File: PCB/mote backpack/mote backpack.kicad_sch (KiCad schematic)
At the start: 15 parts, among them J1 DF17_2.0_-30DP-0.5V_57_, J2 73251-1350, J3 Micro_SD_Card_Det2, J4 Conn_01x06_Socket, U1 MAX3232, U3 ADAFRUIT_QT_PY

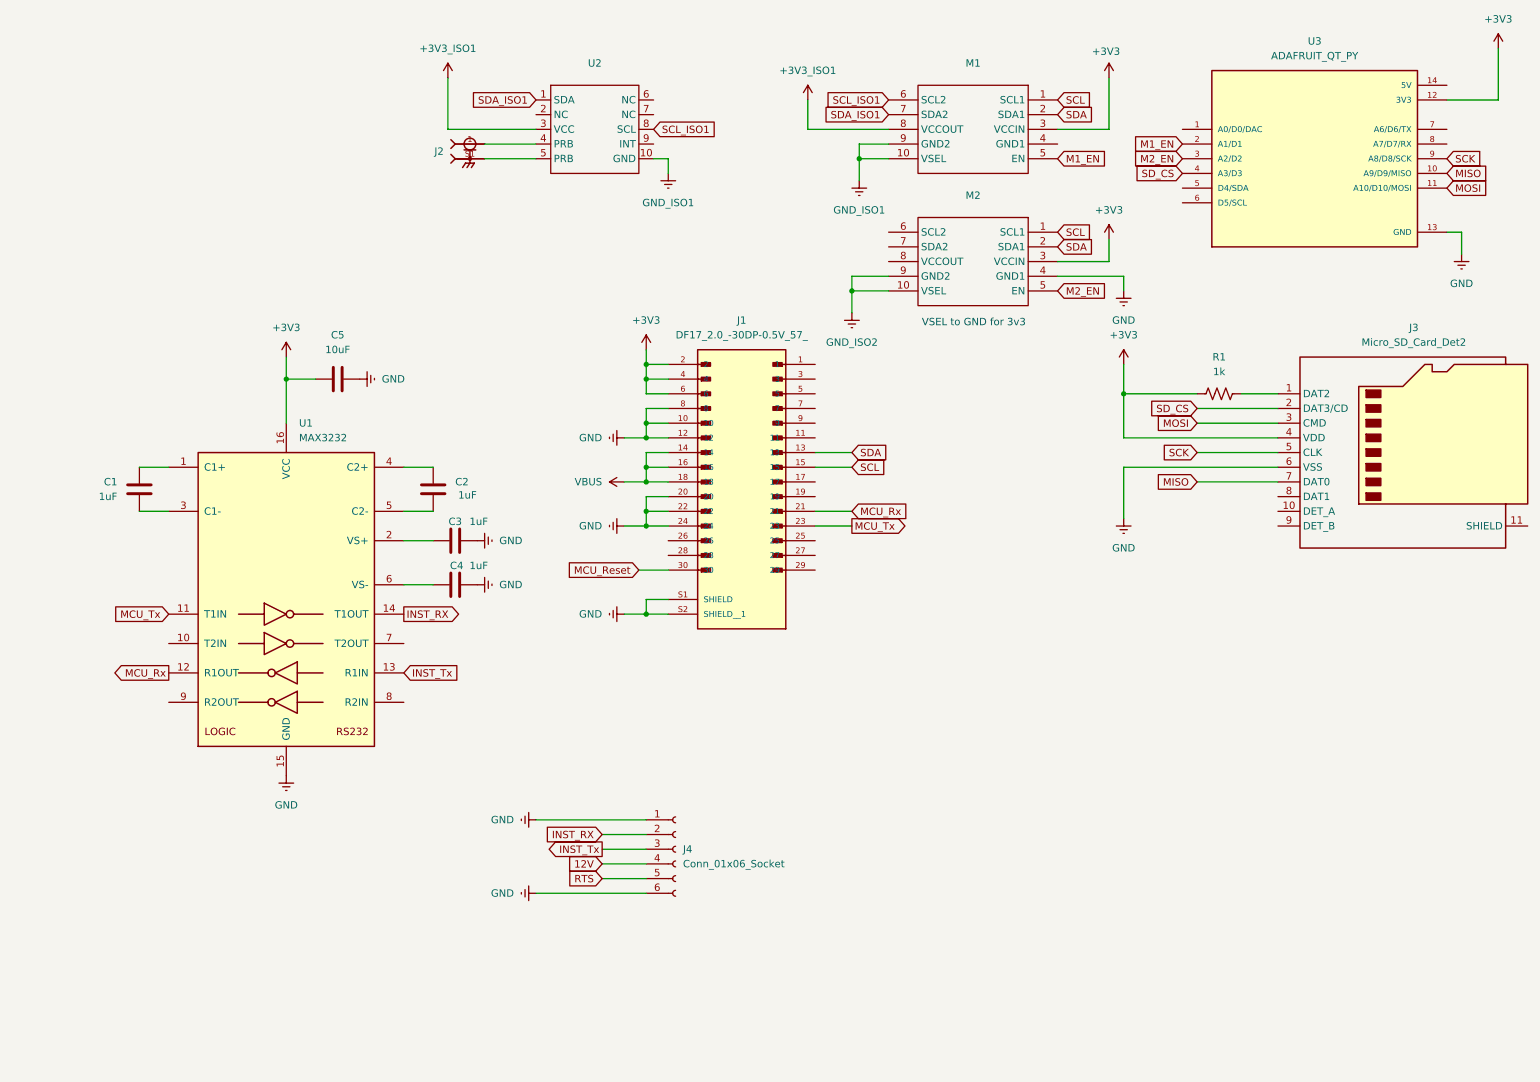
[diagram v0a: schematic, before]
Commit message: test that changes tracked
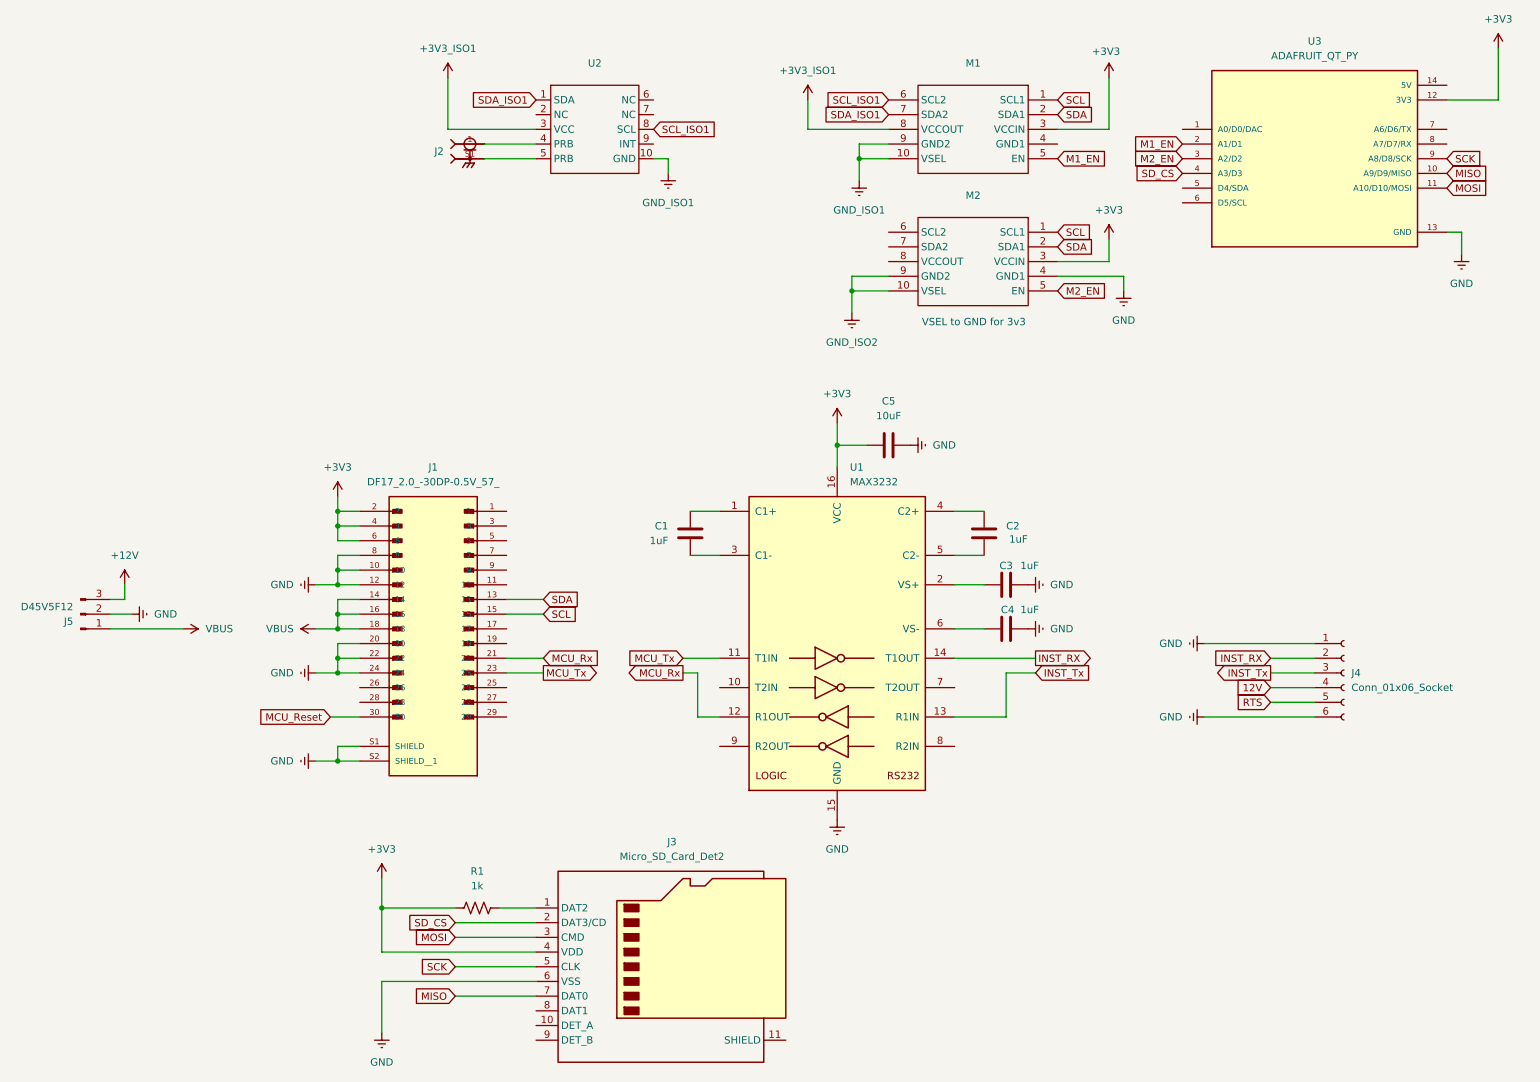
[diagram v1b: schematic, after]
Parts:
- added J5: D45V5F12, Connector_PinHeader_2.54mm:PinHeader_1x03_P2.54mm_Vertical, symbol Connector:Conn_01x03_Pin
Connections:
- net GND: now also J5.2 (Pin_2)
- net VBUS: now also J5.1 (Pin_1)
- new net +12V: J5.3 (Pin_3)
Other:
- moved on the sheet: C1, C2, C3, C4, C5, J1, J3, J4, R1, U1
